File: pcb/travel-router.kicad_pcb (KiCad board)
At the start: 4 copper layers, 100 x 100 mm, 54 parts, among them J1 USB_C_Receptacle_USB2.0_14P, J2 Conn_02x05_Odd_Even, J6 JST_SHBM048-SRSS-TB, J8 USB_A_Stacked, SW1 SW_Push, U1 RT9742SNGV, U10 TPD4EUSB30, U11 TPD2E2U06DCK, U12 476591100, U2 AP2553W6, U3 MagJack-A70-112-331N126, U4 TPD4EUSB30, U5 TPD4EUSB30, U6 RTL8111H-CG, U7 MagJack-A70-112-331N126, U8 TPD4EUSB30, U9 TPD4EUSB30, Y1 XL2EL89COI-111YLC-25M

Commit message: Create README.md
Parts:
- R2, R3: value 1k -> 1K
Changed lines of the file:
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@@
 			)
 		)
-		(property "Value" "1k"
+		(property "Value" "1K"
 			(at 0 1.17 0)
 			(layer "F.Fab")
@@
 			)
 		)
-		(property "Value" "1k"
+		(property "Value" "1K"
 			(at 0 1.17 0)
 			(layer "F.Fab")

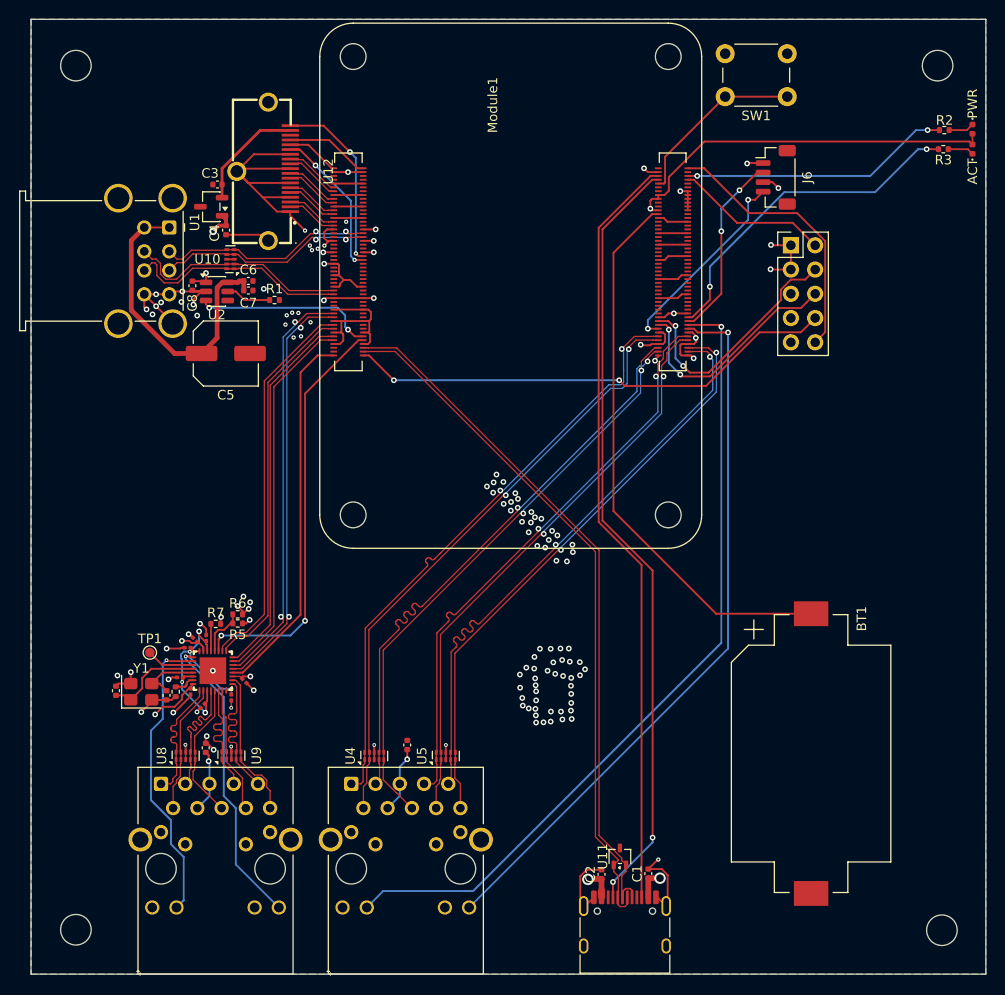
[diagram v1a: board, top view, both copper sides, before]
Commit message: pcb stuff
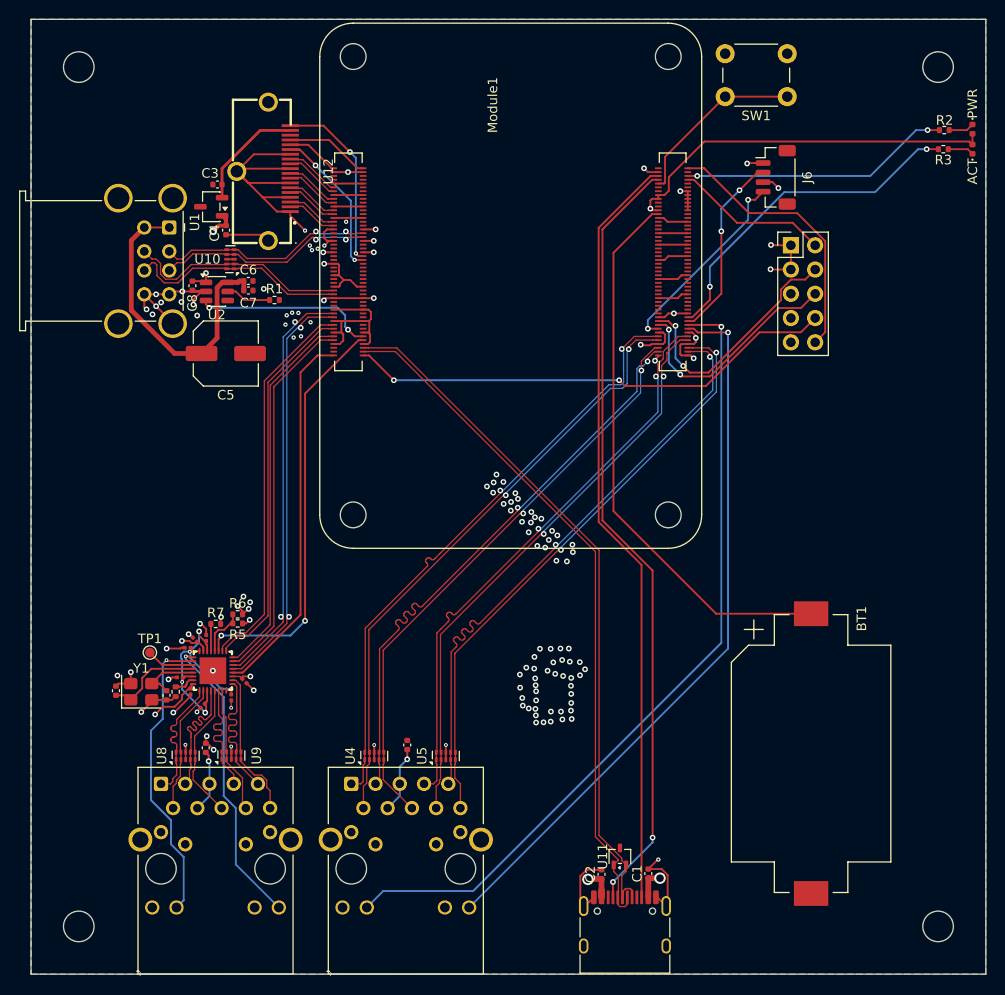
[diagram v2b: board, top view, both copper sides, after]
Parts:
- moved H4 0.57 mm to (183.3, 142.9)
- moved H3 0.46 mm to (93.3, 142.9)
- moved H1 0.34 mm to (93.3, 52.9)
- moved H2 0.16 mm to (183.3, 52.9)
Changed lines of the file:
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@@
 	(footprint "MountingHole:MountingHole_3.2mm_M3"
 		(layer "F.Cu")
-		(at 183.7 143.3)
+		(at 183.3 142.9)
 		(descr "Mounting Hole 3.2mm, M3, no annular, generated by kicad-footprint-generator mountinghole.py")
 		(tags "mountinghole M3")
@@
 		)
 		(embedded_fonts no)
-		(model "${KICAD10_3DMODEL_DIR}/Connector_USB.3dshapes/USB_C_Receptacle_HRO_TYPE-C-31-M-12.step"
-			(offset
-				(xyz 0 0 0)
-			)
-			(scale
-				(xyz 1 1 1)
-			)
-			(rotate
-				(xyz 0 0 0)
-			)
-		)
 		(model "${KICAD10_3DMODEL_DIR}/Connector_USB.3dshapes/USB_C_Receptacle_GCT_USB4105-xx-A_16P_TopMnt_Horizontal.step"
 			(offset
@@
 	(footprint "MountingHole:MountingHole_3.2mm_M3"
 		(layer "F.Cu")
-		(at 183.25 52.75)
+		(at 183.3 52.9)
 		(descr "Mounting Hole 3.2mm, M3, no annular, generated by kicad-footprint-generator mountinghole.py")
 		(tags "mountinghole M3")
@@
 	(footprint "MountingHole:MountingHole_3.2mm_M3"
 		(layer "F.Cu")
-		(at 93 143.25)
+		(at 93.3 142.9)
 		(descr "Mounting Hole 3.2mm, M3, no annular, generated by kicad-footprint-generator mountinghole.py")
 		(tags "mountinghole M3")
@@
 	(footprint "MountingHole:MountingHole_3.2mm_M3"
 		(layer "F.Cu")
-		(at 93 52.75)
+		(at 93.3 52.9)
 		(descr "Mounting Hole 3.2mm, M3, no annular, generated by kicad-footprint-generator mountinghole.py")
 		(tags "mountinghole M3")
